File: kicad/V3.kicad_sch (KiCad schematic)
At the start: 5 parts

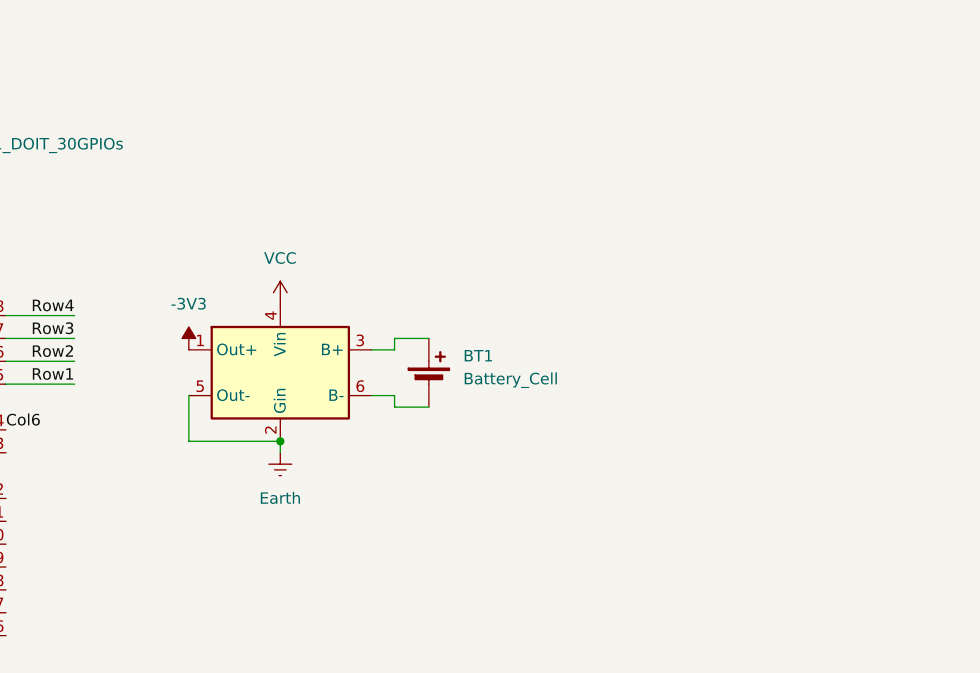
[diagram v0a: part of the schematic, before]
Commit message: switch
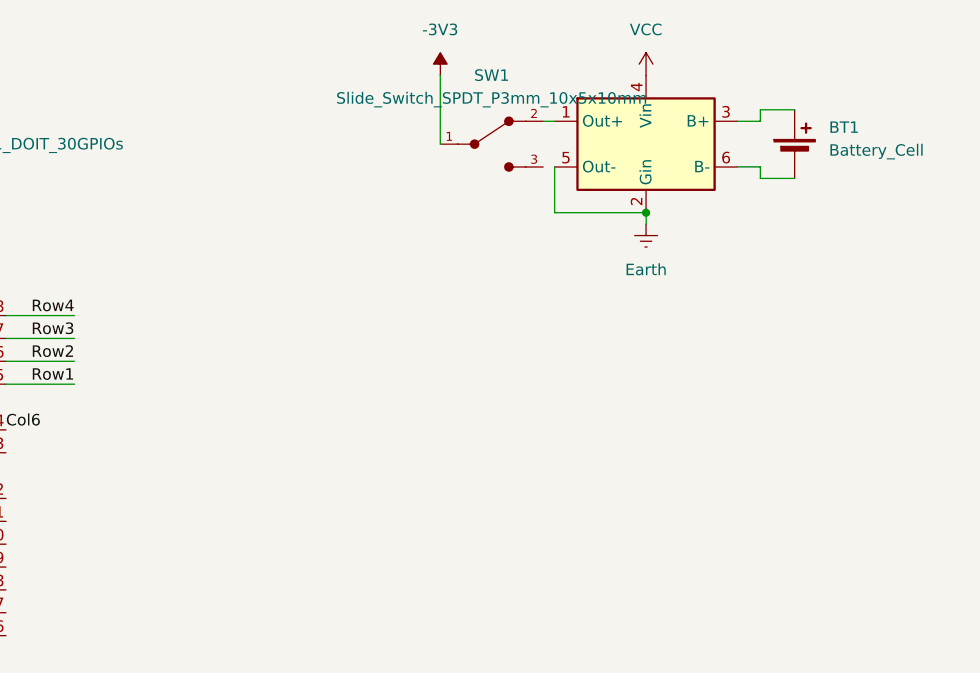
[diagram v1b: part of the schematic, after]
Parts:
- added SW1: Slide_Switch_SPDT_P3mm_10x5x10mm, PCM_SL_Devices:Slide_Switch_SPDT_P3mm_10x5x10mm, symbol PCM_SL_Devices:Slide_Switch_SPDT_P3mm_10x5x10mm
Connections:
- net -3V3: now also SW1.1; no longer U1.1 (Out+)
- new net: SW1.2, U1.1 (Out+)
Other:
- moved on the sheet: BT1
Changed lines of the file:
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@@
 	)
 	(junction
-		(at 218.44 64.77)
+		(at 259.08 39.37)
 		(diameter 0)
 		(color 0 0 0 0)
@@
 	(wire
 		(pts
-			(xy 231.14 53.34) (xy 234.95 53.34)
+			(xy 271.78 27.94) (xy 275.59 27.94)
 		)
 		(stroke
@@
 	(wire
 		(pts
+			(xy 247.65 29.21) (xy 248.92 29.21)
+		)
+		(stroke
+			(width 0)
+			(type default)
+		)
+	)
+	(wire
+		(pts
 			(xy 80.01 50.8) (xy 80.01 72.39)
 		)
@@
 	(wire
 		(pts
-			(xy 218.44 66.04) (xy 218.44 64.77)
+			(xy 259.08 40.64) (xy 259.08 39.37)
 		)
 		(stroke
@@
 	(wire
 		(pts
-			(xy 231.14 53.34) (xy 231.14 54.61)
+			(xy 271.78 27.94) (xy 271.78 29.21)
 		)
 		(stroke
@@
 	(wire
 		(pts
-			(xy 208.28 64.77) (xy 218.44 64.77)
+			(xy 248.92 39.37) (xy 259.08 39.37)
 		)
 		(stroke
@@
 	(wire
 		(pts
-			(xy 208.28 59.69) (xy 208.28 64.77)
+			(xy 248.92 34.29) (xy 248.92 39.37)
 		)
 		(stroke
@@
 	(wire
 		(pts
-			(xy 231.14 60.96) (xy 231.14 59.69)
+			(xy 271.78 35.56) (xy 271.78 34.29)
 		)
 		(stroke
@@
 	(wire
 		(pts
-			(xy 228.6 54.61) (xy 231.14 54.61)
+			(xy 269.24 29.21) (xy 271.78 29.21)
 		)
 		(stroke
@@
 	(wire
 		(pts
-			(xy 231.14 60.96) (xy 234.95 60.96)
+			(xy 271.78 35.56) (xy 275.59 35.56)
 		)
 		(stroke
@@
 	(wire
 		(pts
-			(xy 228.6 59.69) (xy 231.14 59.69)
+			(xy 269.24 34.29) (xy 271.78 34.29)
+		)
+		(stroke
+			(width 0)
+			(type default)
+		)
+	)
+	(wire
+		(pts
+			(xy 236.22 31.75) (xy 236.22 24.13)
 		)
 		(stroke
@@
 	(symbol
 		(lib_id "Library:TP4056_usb_module")
-		(at 215.9 55.88 0)
+		(at 256.54 30.48 0)
 		(unit 1)
 		(exclude_from_sim no)
@@
 		(fields_autoplaced yes)
 		(property "Reference" "U1"
-			(at 214.63 57.15 90)
+			(at 255.27 31.75 90)
 			(effects
 				(font
@@
 		)
 		(property "Value" "~"
-			(at 220.5833 50.8 0)
+			(at 261.2233 25.4 0)
 			(effects
 				(font
@@
 		)
 		(property "Footprint" "Library:HAYATEC TP4056 LIPO CHARGING MODULE"
-			(at 215.9 55.88 0)
+			(at 256.54 30.48 0)
 			(effects
 				(font
@@
 		)
 		(property "Datasheet" ""
-			(at 215.9 55.88 0)
+			(at 256.54 30.48 0)
 			(effects
 				(font
@@
 		)
 		(property "Description" ""
-			(at 215.9 55.88 0)
+			(at 256.54 30.48 0)
 			(effects
 				(font
@@
 	(symbol
 		(lib_id "power:Earth")
-		(at 218.44 66.04 0)
+		(at 259.08 40.64 0)
 		(unit 1)
 		(exclude_from_sim no)
@@
 		(fields_autoplaced yes)
 		(property "Reference" "#PWR01"
-			(at 218.44 72.39 0)
+			(at 259.08 46.99 0)
 			(effects
 				(font
@@
 		)
 		(property "Value" "Earth"
-			(at 218.44 71.12 0)
+			(at 259.08 45.72 0)
 			(effects
 				(font
@@
 		)
 		(property "Footprint" ""
-			(at 218.44 66.04 0)
+			(at 259.08 40.64 0)
 			(effects
 				(font
@@
 		)
 		(property "Datasheet" "~"
-			(at 218.44 66.04 0)
+			(at 259.08 40.64 0)
 			(effects
 				(font
@@
 		)
 		(property "Description" "Power symbol creates a global label with name \"Earth\""
-			(at 218.44 66.04 0)
+			(at 259.08 40.64 0)
 			(effects
 				(font
@@
 	)
 	(symbol
+		(lib_id "PCM_SL_Devices:Slide_Switch_SPDT_P3mm_10x5x10mm")
+		(at 242.57 31.75 0)
+		(unit 1)
+		(exclude_from_sim no)
+		(in_bom yes)
+		(on_board yes)
+		(dnp no)
+		(fields_autoplaced yes)
+		(property "Reference" "SW1"
+			(at 241.935 24.13 0)
+			(effects
+				(font
+					(size 1.27 1.27)
+				)
+			)
+		)
+		(property "Value" "Slide_Switch_SPDT_P3mm_10x5x10mm"
+			(at 241.935 26.67 0)
+			(effects
+				(font
+					(size 1.27 1.27)
+				)
+			)
+		)
+		(property "Footprint" "PCM_SL_Devices:Slide_Switch_SPDT_P3mm_10x5x10mm"
+			(at 243.84 39.37 0)
+			(effects
+				(font
+					(size 1.27 1.27)
+				)
+				(hide yes)
+			)
+		)
+		(property "Datasheet" ""
+			(at 241.3 25.4 0)
+			(effects
+				(font
+					(size 1.27 1.27)
+				)
+				(hide yes)
+			)
+		)
+		(property "Description" "SPDT Slide Switch with 10mm length, 5mm width and 10mm hight."
+			(at 242.57 31.75 0)
+			(effects
+				(font
+					(size 1.27 1.27)
+				)
+				(hide yes)
+			)
+		)
+		(pin "2"
+		)
+		(pin "3"
+		)
+		(pin "1"
+		)
+		(instances
+			(project ""
+				(path "/55ac274f-6d39-4edb-ae03-cf051723ec39"
+					(reference "SW1")
+					(unit 1)
+				)
+			)
+		)
+	)
+	(symbol
 		(lib_id "power:VCC")
-		(at 218.44 49.53 0)
+		(at 259.08 24.13 0)
 		(unit 1)
 		(exclude_from_sim no)
@@
 		(fields_autoplaced yes)
 		(property "Reference" "#PWR03"
-			(at 218.44 53.34 0)
+			(at 259.08 27.94 0)
 			(effects
 				(font
@@
 		)
 		(property "Value" "VCC"
-			(at 218.44 44.45 0)
+			(at 259.08 19.05 0)
 			(effects
 				(font
@@
 		)
 		(property "Footprint" ""
-			(at 218.44 49.53 0)
+			(at 259.08 24.13 0)
 			(effects
 				(font
@@
 		)
 		(property "Datasheet" ""
-			(at 218.44 49.53 0)
+			(at 259.08 24.13 0)
 			(effects
 				(font
@@
 		)
 		(property "Description" "Power symbol creates a global label with name \"VCC\""
-			(at 218.44 49.53 0)
+			(at 259.08 24.13 0)
 			(effects
 				(font
@@
 	(symbol
 		(lib_id "Device:Battery_Cell")
-		(at 234.95 58.42 0)
+		(at 275.59 33.02 0)
 		(unit 1)
 		(exclude_from_sim no)
@@
 		(fields_autoplaced yes)
 		(property "Reference" "BT1"
-			(at 238.76 55.3084 0)
+			(at 279.4 29.9084 0)
 			(effects
 				(font
@@
 		)
 		(property "Value" "Battery_Cell"
-			(at 238.76 57.8484 0)
+			(at 279.4 32.4484 0)
 			(effects
 				(font
@@
 		)
 		(property "Footprint" ""
-			(at 234.95 56.896 90)
+			(at 275.59 31.496 90)
 			(effects
 				(font
@@
 		)
 		(property "Datasheet" "~"
-			(at 234.95 56.896 90)
+			(at 275.59 31.496 90)
 			(effects
 				(font
@@
 		)
 		(property "Description" "Single-cell battery"
-			(at 234.95 58.42 0)
+			(at 275.59 33.02 0)
 			(effects
 				(font
@@
 	(symbol
 		(lib_id "power:-3V3")
-		(at 208.28 54.61 0)
+		(at 236.22 24.13 0)
 		(unit 1)
 		(exclude_from_sim no)
@@
 		(fields_autoplaced yes)
 		(property "Reference" "#PWR08"
-			(at 208.28 58.42 0)
+			(at 236.22 27.94 0)
 			(effects
 				(font
@@
 		)
 		(property "Value" "-3V3"
-			(at 208.28 49.53 0)
+			(at 236.22 19.05 0)
 			(effects
 				(font
@@
 		)
 		(property "Footprint" ""
-			(at 208.28 54.61 0)
+			(at 236.22 24.13 0)
 			(effects
 				(font
@@
 		)
 		(property "Datasheet" ""
-			(at 208.28 54.61 0)
+			(at 236.22 24.13 0)
 			(effects
 				(font
@@
 		)
 		(property "Description" "Power symbol creates a global label with name \"-3V3\""
-			(at 208.28 54.61 0)
-			(effects
-				(font
+			(at 236.22 24.13 0)
+			(effects
+				(font
